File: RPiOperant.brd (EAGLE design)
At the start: 87.3 x 64.8 mm, 31 parts, among them IC1 74LS14N, IC3 MCP3008, J2 POWER_JACK, J3 POWER_JACK

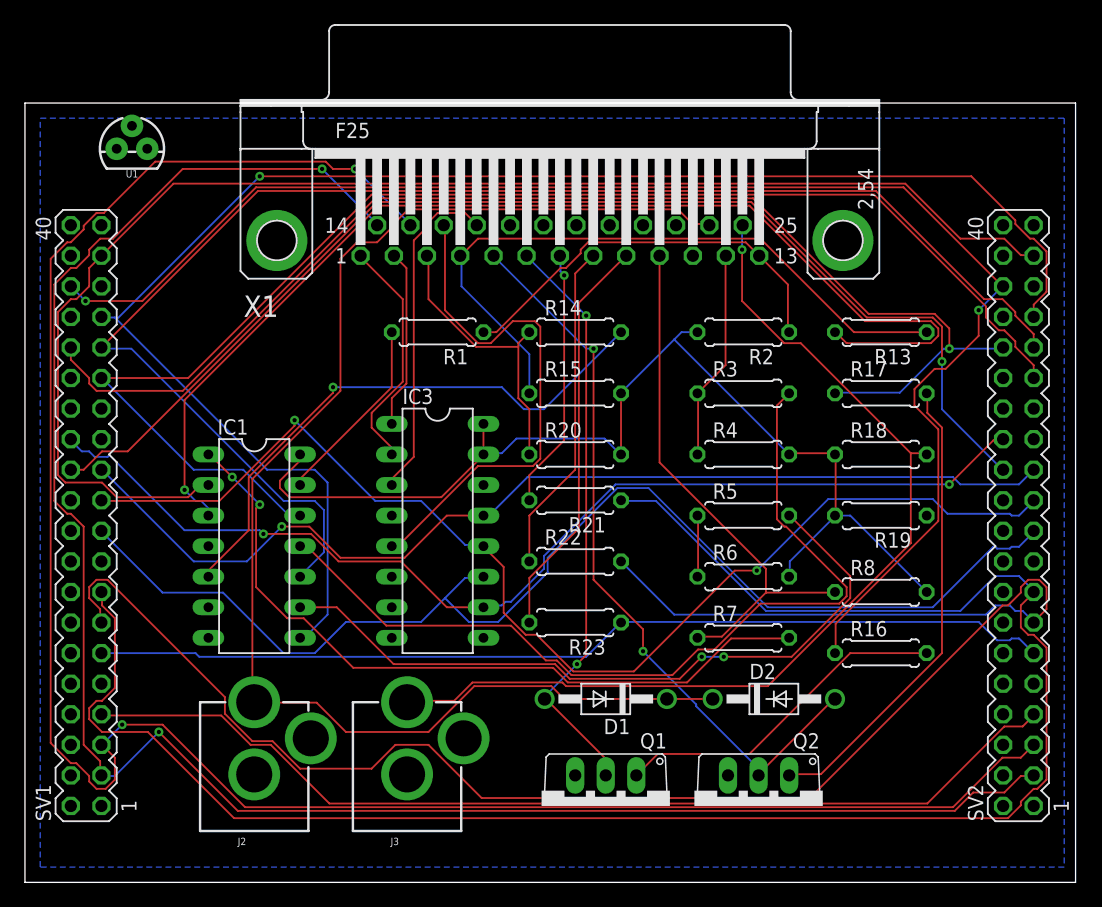
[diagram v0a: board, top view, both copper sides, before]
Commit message: updates
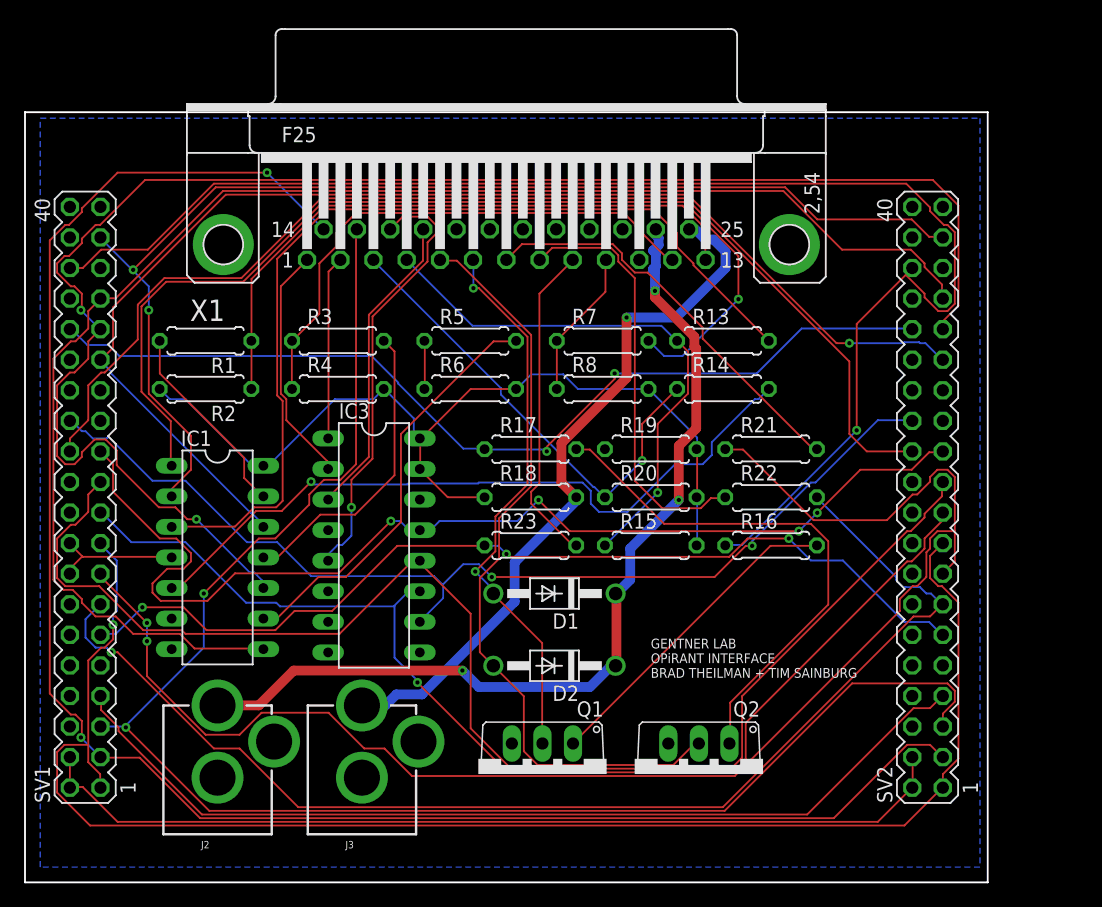
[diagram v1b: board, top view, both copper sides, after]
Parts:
- removed U1: (no value), SparkFun-Sensors:TO-92
- moved R2 44.9 mm to (15.0, 41.0)
- moved R4 34.1 mm to (26.0, 41.0)
- moved R3 34.0 mm to (26.0, 45.0)
- moved R17 29.5 mm to (42.0, 36.0)
- moved R18 29.3 mm to (42.0, 32.0)
- moved R8 28.6 mm to (48.0, 41.0)
- moved R6 27.5 mm to (37.0, 41.0)
- moved R7 27.3 mm to (48.0, 45.0)
- moved R5 26.9 mm to (37.0, 45.0)
- moved R19 19.9 mm to (52.0, 36.0), turned to 0 degrees
- moved R1 19.3 mm to (15.0, 45.0)
- moved D2 18.4 mm to (44.0, 18.0), turned to 180 degrees
- moved R22 17.1 mm to (62.0, 32.0)
- moved R21 16.8 mm to (62.0, 36.0), turned to 0 degrees
- moved R15 14.1 mm to (52.0, 28.0)
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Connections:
- new net RPI_3.3V: SV1.1, SV1.17, SV2.1, SV2.17
- new net RPI_5V: SV1.2, SV1.4, SV2.2, SV2.4
- net IR_1_GPIO: now also SV1.16
- net IR_2_GPIO: now also SV1.18, SV2.18
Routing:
- net RPI_3.3V: track 0.00 -> 127.1 mm, vias 0 -> 1
- net RPI_5V: track 0.00 -> 77.5 mm
- net N$8: track 72.4 -> 25.3 mm
- net GPIO27: track 141.6 -> 101.7 mm, vias 0 -> 1
- net 12V: track 114.1 -> 76.7 mm, vias 0 -> 3
- net GPIO3: track 169.9 -> 132.9 mm
- net RIGHT_IR: track 44.7 -> 12.4 mm
- net GPIO22: track 153.8 -> 125.1 mm, vias 0 -> 2
- net LEFT_IR: track 17.5 -> 44.8 mm
- net N$10: track 60.0 -> 34.9 mm, vias 2 -> 0
- net LIGHTS_TRIG_GPIO: track 103.7 -> 79.0 mm, vias 1 -> 2
- net +5V: track 82.0 -> 59.9 mm
- net N$12: track 62.2 -> 83.0 mm, vias 2 -> 1
- net RIGHT_PECK_GPIO: track 116.2 -> 97.2 mm, vias 0 -> 2
- net HOPPER_IR: track 34.1 -> 52.8 mm
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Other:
- board size 87.3 x 64.8 mm -> 80 x 64 mm
- board text added: "GENTNER LAB OPiRANT INTERFACE BRAD THEILMAN + TIM SAINBURG"
